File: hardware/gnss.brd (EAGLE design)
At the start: 33.5 x 34.6 mm, 39 parts, among them J1 MICRO_USB_B_HIROSE_ZX62-B-5PA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, SW1 TVAF06-A020B-R, U2 NJM12888F, X1 FA-238

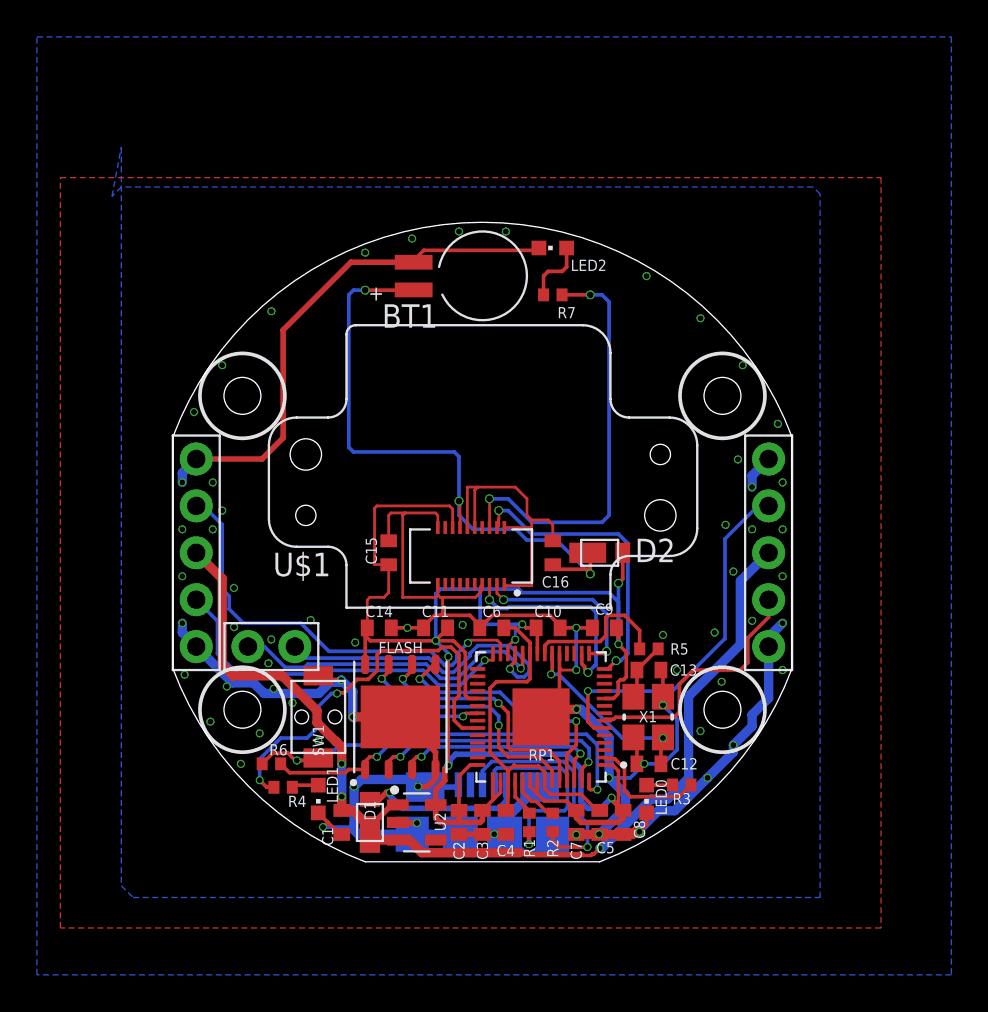
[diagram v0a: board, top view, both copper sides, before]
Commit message: 微修正
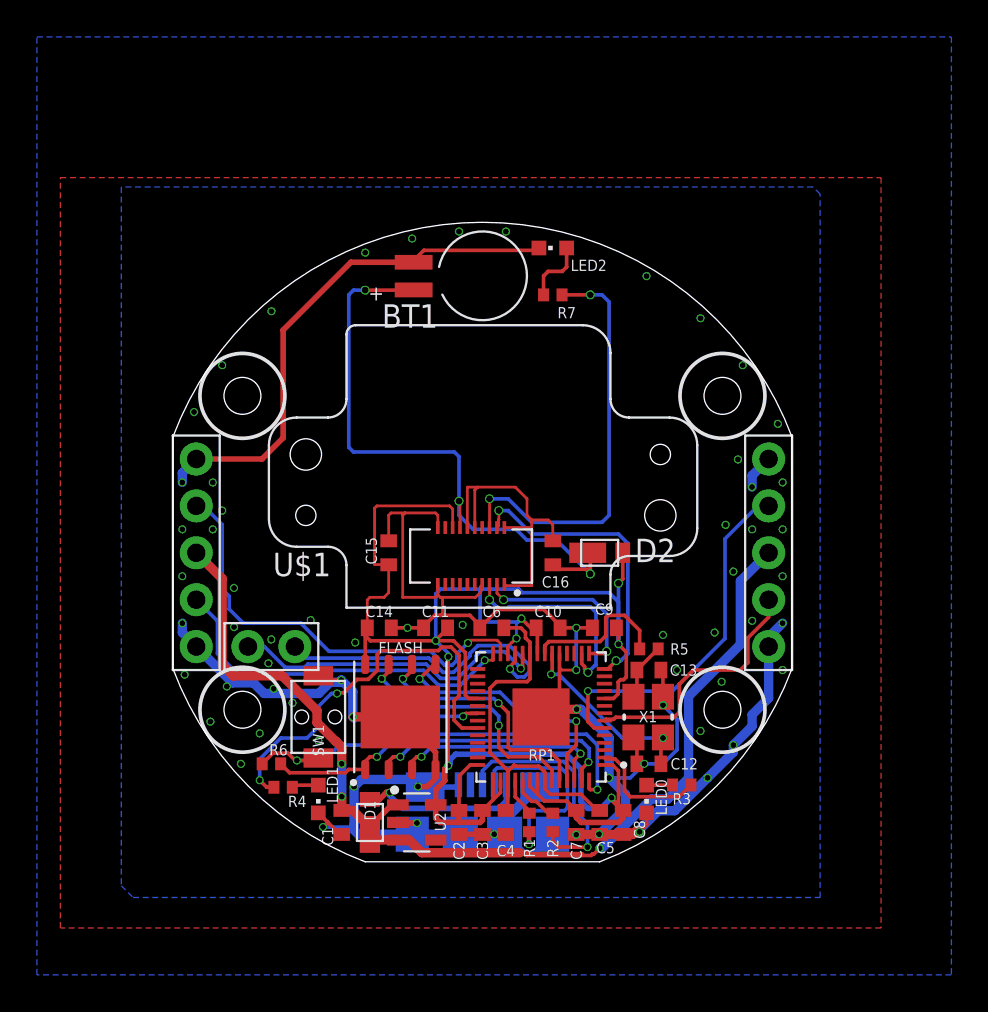
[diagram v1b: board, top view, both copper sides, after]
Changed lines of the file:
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@@
 <wire x1="-2.53" y1="-4.763" x2="-1.57" y2="-4.763" width="0.2" layer="1"/>
 <wire x1="-1.57" y1="-4.763" x2="-0.9235" y2="-5.4095" width="0.2" layer="1"/>
-<wire x1="2.906" y1="-4.064" x2="2.35" y2="-4.064" width="0.2" layer="1"/>
-<wire x1="2.35" y1="-4.064" x2="2.159" y2="-3.873" width="0.2" layer="1"/>
-<via x="2.159" y="-3.873" extent="1-16" drill="0.3"/>
+<wire x1="2.906" y1="-4.064" x2="2.615" y2="-4.064" width="0.2" layer="1"/>
+<wire x1="2.615" y1="-4.064" x2="2.1105" y2="-3.5595" width="0.2" layer="1"/>
+<via x="2.1105" y="-3.5595" extent="1-16" drill="0.3"/>
 <wire x1="-2.53" y1="-2.223" x2="-2.275" y2="-1.968" width="0.2" layer="16"/>
 <wire x1="-2.53" y1="-2.223" x2="-2.53" y2="-4.763" width="0.2" layer="16"/>
@@
 <wire x1="0" y1="-1.968" x2="-0.127" y2="-2.095" width="0.2" layer="16"/>
 <wire x1="-0.127" y1="-2.095" x2="-0.127" y2="-3.683" width="0.2" layer="16"/>
-<wire x1="-0.127" y1="-3.683" x2="0.063" y2="-3.873" width="0.2" layer="16"/>
-<wire x1="0.063" y1="-3.873" x2="2.159" y2="-3.873" width="0.2" layer="16"/>
+<wire x1="-0.127" y1="-3.683" x2="-0.063" y2="-3.747" width="0.2" layer="16"/>
+<wire x1="1.923" y1="-3.747" x2="-0.063" y2="-3.747" width="0.2" layer="16"/>
+<wire x1="1.923" y1="-3.747" x2="2.1105" y2="-3.5595" width="0.2" layer="16"/>
 <wire x1="7.3495" y1="-7.6365" x2="7.3495" y2="-7.003975" width="0.2" layer="1"/>
 <wire x1="7.3495" y1="-7.003975" x2="7.482475" y2="-6.871" width="0.2" layer="1"/>
@@
 <wire x1="7.096" y1="-7.89" x2="7.3495" y2="-7.6365" width="0.2" layer="1"/>
 <contactref element="RP1" pad="26"/>
-<via x="1.778" y="-4.7" extent="1-16" drill="0.3"/>
+<via x="1.841" y="-4.637" extent="1-16" drill="0.3"/>
 <wire x1="1.605475" y1="-4.8318" x2="1.6462" y2="-4.8318" width="0.1524" layer="1"/>
-<wire x1="1.6462" y1="-4.8318" x2="1.778" y2="-4.7" width="0.1524" layer="1"/>
+<wire x1="1.6462" y1="-4.8318" x2="1.841" y2="-4.637" width="0.1524" layer="1"/>
 <wire x1="1.375" y1="-5.455" x2="1.375" y2="-5.062275" width="0.1524" layer="1"/>
 <wire x1="1.375" y1="-5.062275" x2="1.605475" y2="-4.8318" width="0.1524" layer="1"/>
-<wire x1="2.159" y1="-3.873" x2="1.778" y2="-4.254" width="0.1524" layer="16"/>
-<wire x1="1.778" y1="-4.254" x2="1.778" y2="-4.7" width="0.1524" layer="16"/>
+<wire x1="2.1105" y1="-3.5595" x2="1.841" y2="-3.829" width="0.1524" layer="16"/>
+<wire x1="1.841" y1="-3.829" x2="1.841" y2="-4.637" width="0.1524" layer="16"/>
 </signal>
 <signal name="GND">
@@
 <wire x1="-3.19" y1="-4.064" x2="-3.19" y2="-3.988975" width="0.2" layer="1"/>
 <wire x1="-2.588025" y1="-3.387" x2="-3.19" y2="-3.988975" width="0.2" layer="1"/>
-<wire x1="-0.142" y1="-4.064" x2="0.535" y2="-3.387" width="0.2" layer="1"/>
-<wire x1="3.641" y1="-3.387" x2="4.318" y2="-4.064" width="0.2" layer="1"/>
-<wire x1="0.535" y1="-3.387" x2="3.641" y2="-3.387" width="0.2" layer="1"/>
+<wire x1="-0.142" y1="-4.064" x2="0.85" y2="-3.072" width="0.2" layer="1"/>
+<wire x1="3.326" y1="-3.072" x2="4.318" y2="-4.064" width="0.2" layer="1"/>
+<wire x1="0.85" y1="-3.072" x2="3.326" y2="-3.072" width="0.2" layer="1"/>
 <wire x1="4.175" y1="-5.455" x2="4.175" y2="-6.223" width="0.2" layer="1"/>
 <wire x1="4.175" y1="-6.223" x2="4.175" y2="-7.89" width="0.2" layer="1"/>
@@
 <wire x1="-0.415" y1="1.366" x2="-0.415" y2="3.395" width="0.1524" layer="1"/>
 <polygon width="0.1524" layer="16">
-<vertex x="-19.558" y="21.971"/>
+<vertex x="-19.558" y="19.812"/>
 <vertex x="-19.558" y="-18.034"/>
 <vertex x="-18.923" y="-18.669"/>
@@
 <vertex x="18.288" y="19.431"/>
 <vertex x="17.907" y="19.812"/>
-<vertex x="-19.558" y="19.812"/>
-<vertex x="-20.066" y="19.304"/>
 </polygon>
-<wire x1="11.811" y1="12.7" x2="14.097" y2="10.16" width="0" layer="19" extent="1-1"/>
-<wire x1="16.002" y1="6.985" x2="14.097" y2="10.16" width="0" layer="19" extent="1-1"/>
-<wire x1="15.5" y1="5.08" x2="16.002" y2="6.985" width="0" layer="19" extent="1-1"/>
-<wire x1="16.256" y1="3.81" x2="15.5" y2="5.08" width="0" layer="19" extent="1-1"/>
-<wire x1="13.8385" y1="5.0585" x2="15.5" y2="5.08" width="0" layer="19" extent="1-1"/>
-<wire x1="14.605" y1="1.27" x2="14.605" y2="3.556" width="0" layer="19" extent="1-1"/>
-<wire x1="13.171" y1="1.511" x2="14.605" y2="1.27" width="0" layer="19" extent="1-1"/>
-<wire x1="16.256" y1="1.27" x2="14.605" y2="1.27" width="0" layer="19" extent="1-1"/>
-<wire x1="13.589" y1="-1.016" x2="14.605" y2="1.27" width="0" layer="19" extent="1-1"/>
-<wire x1="16.256" y1="-1.27" x2="16.256" y2="1.27" width="0" layer="19" extent="1-1"/>
-<wire x1="16.256" y1="-3.81" x2="16.256" y2="-1.27" width="0" layer="19" extent="1-1"/>
-<wire x1="6.3165" y1="-15.241" x2="6.35" y2="-15.255" width="0" layer="19" extent="1-1"/>
-<wire x1="-1.27" y1="-15.255" x2="-1.2" y2="-15.24" width="0" layer="19" extent="1-16"/>
-<wire x1="-3.49" y1="-12.6605" x2="-3.1" y2="-12.69" width="0" layer="19" extent="16-16"/>
-<wire x1="0.635" y1="-15.24" x2="1.2" y2="-15.24" width="0" layer="19" extent="16-16"/>
-<wire x1="10.541" y1="-6.35" x2="9.667" y2="-6.35" width="0" layer="19" extent="1-1"/>
-<wire x1="5.954" y1="-4.064" x2="5.08" y2="-4.064" width="0" layer="19" extent="1-1"/>
-<wire x1="-1.071" y1="-3.906" x2="-0.142" y2="-4.064" width="0" layer="19" extent="1-1"/>
-<wire x1="1.185" y1="-1.714" x2="-0.015" y2="-1.714" width="0" layer="19" extent="1-1"/>
-<wire x1="16.256" y1="-6.35" x2="15.5" y2="-5.08" width="0" layer="19" extent="1-1"/>
-<wire x1="-16.129" y1="-6.604" x2="-15.5" y2="-5.08" width="0" layer="19" extent="1-1"/>
-<wire x1="14.605" y1="-3.683" x2="16.256" y2="-3.81" width="0" layer="19" extent="1-1"/>
-<wire x1="9.779" y1="-4.445" x2="9.667" y2="-6.35" width="0" layer="19" extent="1-1"/>
-<wire x1="11.811" y1="-9.652" x2="13.589" y2="-10.414" width="0" layer="19" extent="1-1"/>
-<wire x1="-10.287" y1="-8.128" x2="-8.89" y2="-6.665" width="0" layer="19" extent="1-1"/>
-<wire x1="-11.303" y1="-7.366" x2="-10.287" y2="-8.128" width="0" layer="19" extent="1-1"/>
-<wire x1="-11.592" y1="-5.985" x2="-11.303" y2="-7.366" width="0" layer="19" extent="1-1"/>
-<wire x1="-11.4345" y1="-4.6935" x2="-11.592" y2="-5.985" width="0" layer="19" extent="1-1"/>
-<wire x1="-13.45" y1="-4.0235" x2="-11.4345" y2="-4.6935" width="0" layer="19" extent="1-1"/>
-<wire x1="-13.462" y1="-1.905" x2="-13.45" y2="-4.0235" width="0" layer="19" extent="1-1"/>
-<wire x1="-6.8895" y1="-4.8605" x2="-4.938" y2="-4.064" width="0" layer="19" extent="1-1"/>
-<wire x1="12.573" y1="-4.318" x2="14.605" y2="-3.683" width="0" layer="19" extent="1-1"/>
-<wire x1="-8.886" y1="-10.1735" x2="-7.0195" y2="-8.89" width="0" layer="19" extent="1-1"/>
-<wire x1="-13.843" y1="-7.239" x2="-16.129" y2="-6.604" width="0" layer="19" extent="1-1"/>
-<wire x1="-14.732" y1="-9.144" x2="-13.843" y2="-7.239" width="0" layer="19" extent="1-1"/>
-<wire x1="-9.3035" y1="-3.6485" x2="-11.4345" y2="-4.6935" width="0" layer="19" extent="1-1"/>
-<wire x1="-12.065" y1="-9.779" x2="-10.287" y2="-8.128" width="0" layer="19" extent="1-1"/>
-<wire x1="-13.081" y1="-11.43" x2="-12.065" y2="-9.779" width="0" layer="19" extent="1-1"/>
-<wire x1="12.954" y1="-6.985" x2="10.541" y2="-6.35" width="0" layer="19" extent="1-1"/>
-<wire x1="-16.256" y1="-1.27" x2="-16.256" y2="-3.81" width="0" layer="19" extent="1-1"/>
-<wire x1="-16.256" y1="1.27" x2="-16.256" y2="-1.27" width="0" layer="19" extent="1-1"/>
-<wire x1="-14.605" y1="1.27" x2="-16.256" y2="1.27" width="0" layer="19" extent="1-1"/>
-<wire x1="-14.097" y1="2.286" x2="-14.605" y2="1.27" width="0" layer="19" extent="1-1"/>
-<wire x1="-14.605" y1="3.81" x2="-14.097" y2="2.286" width="0" layer="19" extent="1-1"/>
-<wire x1="-15.5" y1="5.08" x2="-14.605" y2="3.81" width="0" layer="19" extent="1-1"/>
-<wire x1="-3.81" y1="17.018" x2="-3.725" y2="15.736" width="0" layer="19" extent="1-1"/>
-<wire x1="1.27" y1="17.399" x2="3.06" y2="16.51" width="0" layer="19" extent="1-1"/>
-<wire x1="-1.27" y1="17.399" x2="1.27" y2="17.399" width="0" layer="19" extent="1-1"/>
-<wire x1="-15.621" y1="7.62" x2="-15.5" y2="5.08" width="0" layer="19" extent="1-1"/>
-<wire x1="-6.35" y1="16.256" x2="-3.81" y2="17.018" width="0" layer="19" extent="1-1"/>
-<wire x1="-14.097" y1="10.16" x2="-15.621" y2="7.62" width="0" layer="19" extent="1-1"/>
-<wire x1="8.89" y1="14.986" x2="11.811" y2="12.7" width="0" layer="19" extent="1-1"/>
-<wire x1="-11.43" y1="13.081" x2="-14.097" y2="10.16" width="0" layer="19" extent="1-1"/>
 </signal>
 <signal name="USB_DM">
@@
 <wire x1="2.575" y1="-6.823" x2="2.575" y2="-5.455" width="0.2" layer="1"/>
 <wire x1="0.4125" y1="-10.8265" x2="0.4125" y2="-7.3345" width="0.2" layer="1"/>
-<wire x1="1.158" y1="-4.064" x2="1.779" y2="-4.064" width="0.2" layer="1"/>
-<wire x1="2.575" y1="-4.86" x2="2.575" y2="-5.455" width="0.2" layer="1"/>
-<wire x1="1.779" y1="-4.064" x2="2.575" y2="-4.86" width="0.2" layer="1"/>
+<wire x1="2.0775" y1="-4.064" x2="2.329" y2="-4.3155" width="0.2" layer="1"/>
+<wire x1="2.329" y1="-4.3155" x2="2.329" y2="-4.608025" width="0.2" layer="1"/>
+<wire x1="2.329" y1="-4.608025" x2="2.575" y2="-4.854025" width="0.2" layer="1"/>
+<wire x1="1.158" y1="-4.064" x2="2.0775" y2="-4.064" width="0.2" layer="1"/>
+<wire x1="2.575" y1="-4.854025" x2="2.575" y2="-5.455" width="0.2" layer="1"/>
 </signal>
 <signal name="N$6">
